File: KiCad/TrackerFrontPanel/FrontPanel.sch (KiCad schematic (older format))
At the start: 5 parts, among them J1 Conn_01x08, J2 Conn_01x20, J3 Conn_02x04_Odd_Even, J4 Conn_01x06, U1 STM32F303V(B-C)Tx_u

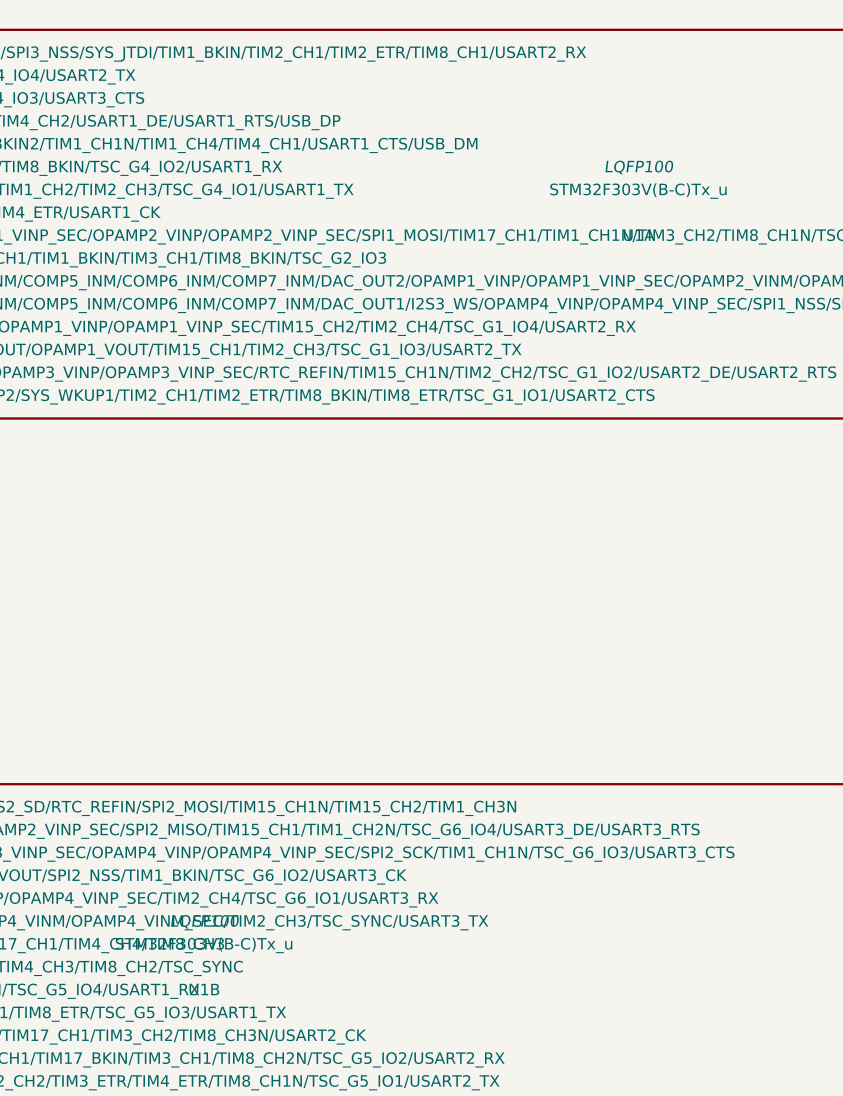
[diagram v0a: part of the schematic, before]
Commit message: save prior to updating to kicad 5
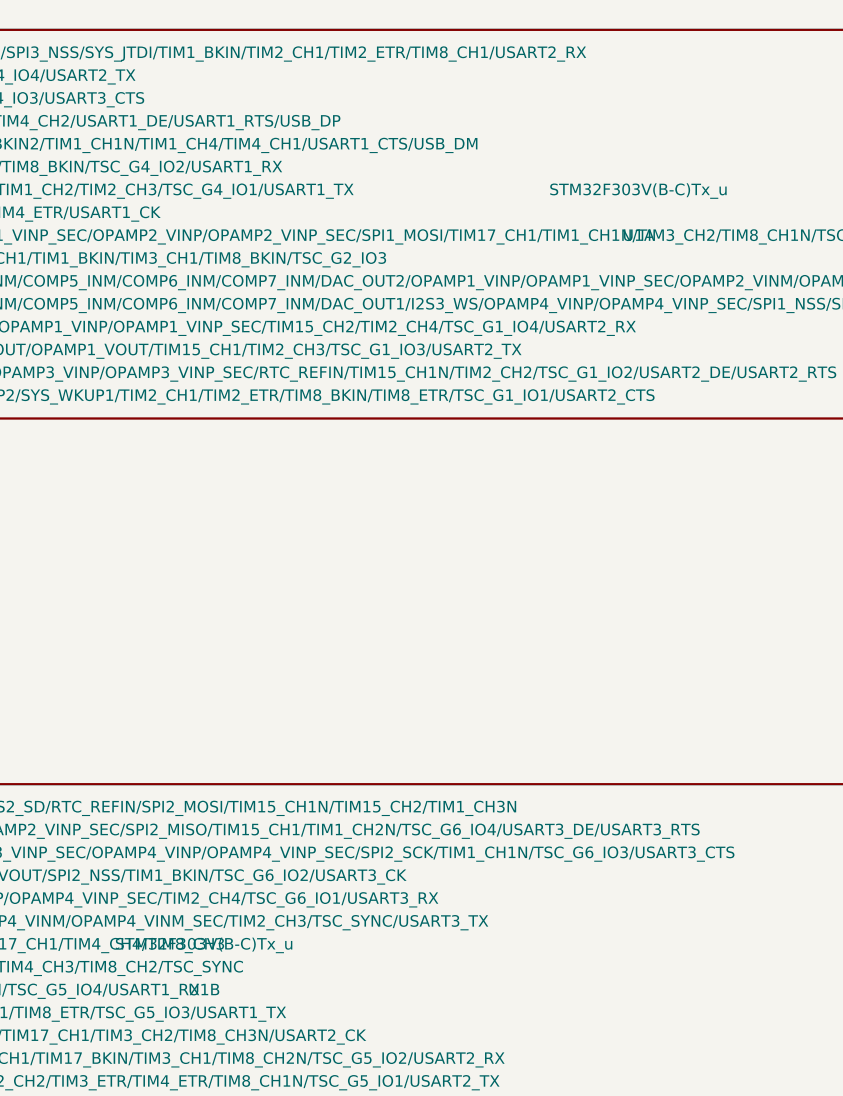
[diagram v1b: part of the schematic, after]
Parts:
- J1: footprint (none) -> footprints:RJ45
- J2: footprint (none) -> Pin_Headers:Pin_Header_Straight_1x20_Pitch2.54mm
- J3: footprint (none) -> Pin_Headers:Pin_Header_Angled_2x04_Pitch2.54mm
- J4: footprint (none) -> Pin_Headers:Pin_Header_Straight_1x06_Pitch2.54mm
- U1: footprint LQFP100 -> Housings_QFP:LQFP-100_14x14mm_Pitch0.5mm
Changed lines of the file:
@@
 F 0 "J2" H 2700 6100 50  0000 C CNN
 F 1 "Conn_01x20" H 2700 4000 50  0000 C CNN
-F 2 "" H 2700 5100 50  0001 C CNN
+F 2 "Pin_Headers:Pin_Header_Straight_1x20_Pitch2.54mm" H 2700 5100 50  0001 C CNN
 F 3 "" H 2700 5100 50  0001 C CNN
 	1    2700 5100
@@
 F 0 "J4" H 5200 7600 50  0000 C CNN
 F 1 "Conn_01x06" H 5200 6900 50  0000 C CNN
-F 2 "" H 5200 7300 50  0001 C CNN
+F 2 "Pin_Headers:Pin_Header_Straight_1x06_Pitch2.54mm" H 5200 7300 50  0001 C CNN
 F 3 "" H 5200 7300 50  0001 C CNN
 	1    5200 7300
@@
 F 0 "J3" H 3750 1200 50  0000 C CNN
 F 1 "Conn_02x04_Odd_Even" H 3750 700 50  0000 C CNN
-F 2 "" H 3700 1000 50  0001 C CNN
+F 2 "Pin_Headers:Pin_Header_Angled_2x04_Pitch2.54mm" H 3700 1000 50  0001 C CNN
 F 3 "" H 3700 1000 50  0001 C CNN
 	1    3700 1000
@@
 F 0 "J1" H 1200 2600 50  0000 C CNN
 F 1 "Conn_01x08" H 1200 1700 50  0000 C CNN
-F 2 "" H 1200 2200 50  0001 C CNN
+F 2 "footprints:RJ45" H 1200 2200 50  0001 C CNN
 F 3 "" H 1200 2200 50  0001 C CNN
 	1    1200 2200
@@
 F 0 "U1" H 11400 1700 50  0000 C CNN
 F 1 "STM32F303V(B-C)Tx_u" H 11400 1500 50  0000 C CNN
-F 2 "LQFP100" H 11400 1400 50  0000 C CIN
+F 2 "Housings_QFP:LQFP-100_14x14mm_Pitch0.5mm" H 11400 1400 50  0001 C CIN
 F 3 "" H 11400 1600 50  0000 C CNN
 	1    11400 1600
@@
 F 0 "U1" H 9500 5000 50  0000 C CNN
 F 1 "STM32F303V(B-C)Tx_u" H 9500 4800 50  0000 C CNN
-F 2 "LQFP100" H 9500 4700 50  0000 C CIN
+F 2 "Housings_QFP:LQFP-100_14x14mm_Pitch0.5mm" H 9500 4700 50  0001 C CIN
 F 3 "" H 9500 4900 50  0000 C CNN
 	2    9500 4900

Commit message: get ready to transfer back to main computer
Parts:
- J1: symbol Conn_01x08 -> FrontPanel-rescue:Conn_01x08
- J2: symbol Conn_01x20 -> FrontPanel-rescue:Conn_01x20
- J3: symbol Conn_02x04_Odd_Even -> FrontPanel-rescue:Conn_02x04_Odd_Even
- J4: symbol Conn_01x06 -> FrontPanel-rescue:Conn_01x06
- U1: symbol STM32F303V(B-C)Tx_u -> stm32:STM32F303V(B-C)Tx_u
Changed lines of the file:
@@
-EESchema Schematic File Version 2
-LIBS:power
-LIBS:device
-LIBS:switches
-LIBS:relays
-LIBS:motors
-LIBS:transistors
-LIBS:conn
-LIBS:linear
-LIBS:regul
-LIBS:74xx
-LIBS:cmos4000
-LIBS:adc-dac
-LIBS:memory
-LIBS:xilinx
-LIBS:microcontrollers
-LIBS:dsp
-LIBS:microchip
-LIBS:analog_switches
-LIBS:motorola
-LIBS:texas
-LIBS:intel
-LIBS:audio
-LIBS:interface
-LIBS:digital-audio
-LIBS:philips
-LIBS:display
-LIBS:cypress
-LIBS:siliconi
-LIBS:opto
-LIBS:atmel
-LIBS:contrib
-LIBS:valves
-LIBS:stm32
-LIBS:MyParts
+EESchema Schematic File Version 4
 LIBS:FrontPanel-cache
-EELAYER 25 0
+EELAYER 26 0
 EELAYER END
 $Descr A4 11693 8268
@@
 $EndDescr
 $Comp
-L Conn_01x20 J2
+L FrontPanel-rescue:Conn_01x20 J2
 U 1 1 5B96B692
 P 2700 5100
@@
 $EndComp
 $Comp
-L Conn_01x06 J4
+L FrontPanel-rescue:Conn_01x06 J4
 U 1 1 5B96B7B2
 P 5200 7300
@@
 $EndComp
 $Comp
-L Conn_02x04_Odd_Even J3
+L FrontPanel-rescue:Conn_02x04_Odd_Even J3
 U 1 1 5B96B85D
 P 3700 1000
@@
 $EndComp
 $Comp
-L GND #PWR01
+L power:GND #PWR01
 U 1 1 5B96B92C
 P 4200 900
@@
 $EndComp
 $Comp
-L +3.3V #PWR02
+L power:+3.3V #PWR02
 U 1 1 5B96B94A
 P 4200 1000
@@
 $EndComp
 $Comp
-L GND #PWR03
+L power:GND #PWR03
 U 1 1 5B96BA03
 P 5400 6900
@@
 NoConn ~ 4900 7100
 $Comp
-L GND #PWR04
+L power:GND #PWR04
 U 1 1 5B96BB70
 P 3100 6000
@@
 $EndComp
 $Comp
-L +3.3V #PWR05
+L power:+3.3V #PWR05
 U 1 1 5B96BB8E
 P 3100 5900
@@
 NoConn ~ 2900 5800
 $Comp
-L GND #PWR06
+L power:GND #PWR06
 U 1 1 5B96BC1B
 P 3100 4100
@@
 TX
 $Comp
-L Conn_01x08 J1
+L FrontPanel-rescue:Conn_01x08 J1
 U 1 1 5B96C9E9
 P 1200 2200
@@
 NB: use only Straight through Ethernet cable-
 $Comp
-L GND #PWR07
+L power:GND #PWR07
 U 1 1 5B96CC13
 P 1600 1850
@@
 $EndComp
 $Comp
-L +3.3V #PWR08
+L power:+3.3V #PWR08
 U 1 1 5B96CC33
 P 1600 2450
@@
 	1400 1800 1600 1800
 Wire Wire Line
-	1600 1800 1600 1900
+	1600 1800 1600 1850
 Wire Wire Line
 	1600 1900 1400 1900
@@
 	1400 2400 1600 2400
 Wire Wire Line
-	1600 2400 1600 2500
+	1600 2400 1600 2450
 Wire Wire Line
 	1600 2500 1400 2500
@@
 $EndSheet
 $Comp
-L STM32F303V(B-C)Tx_u U1
+L stm32:STM32F303V(B-C)Tx_u U1
 U 1 1 5B96D604
 P 11400 1600
@@
 $EndComp
 $Comp
-L STM32F303V(B-C)Tx_u U1
+L stm32:STM32F303V(B-C)Tx_u U1
 U 2 1 5B96D829
 P 9500 4900
@@
 NoConn ~ 4000 1100
 NoConn ~ 4000 1200
+Wire Wire Line
+	1600 1850 1600 1900
+Wire Wire Line
+	1600 2450 1600 2500
 $EndSCHEMATC
